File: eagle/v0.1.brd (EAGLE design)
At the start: 20 x 62.2 mm, 12 parts, among them IC1 74LS595N

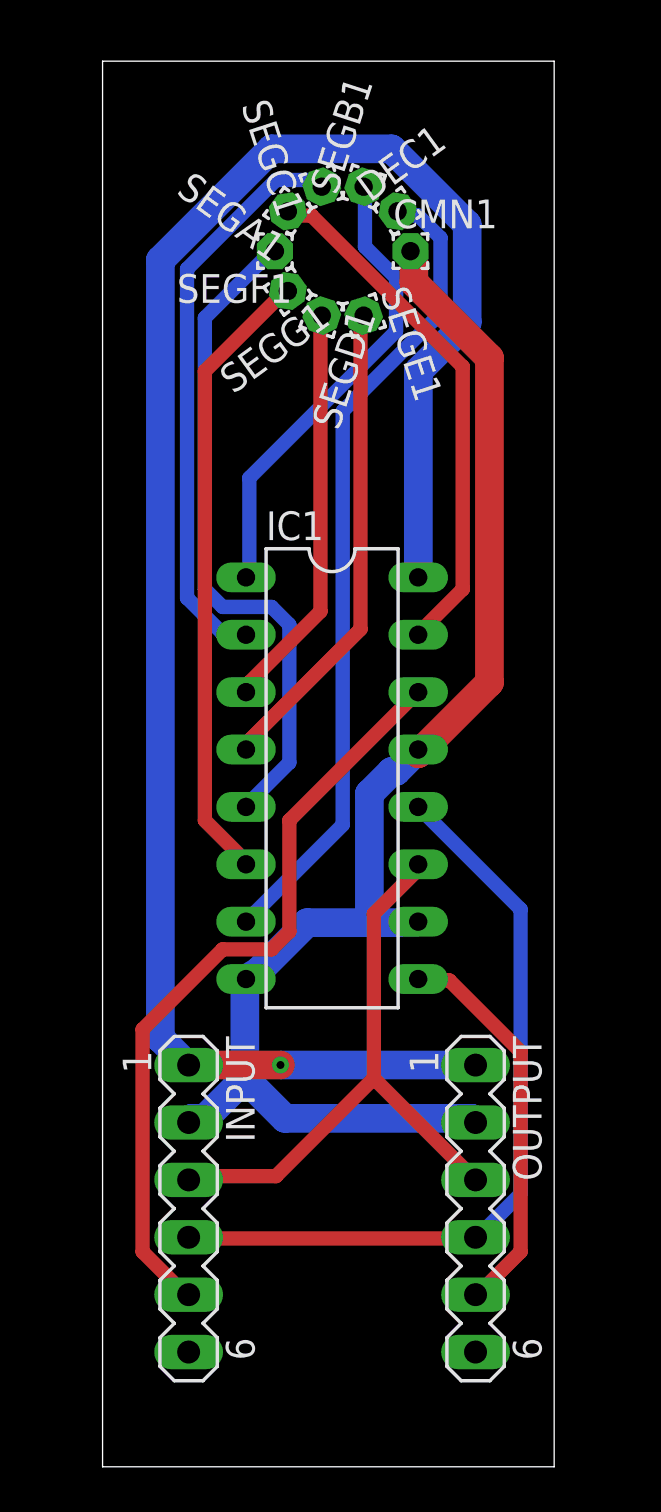
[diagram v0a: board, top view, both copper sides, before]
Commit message: v0.1 as sent to fab
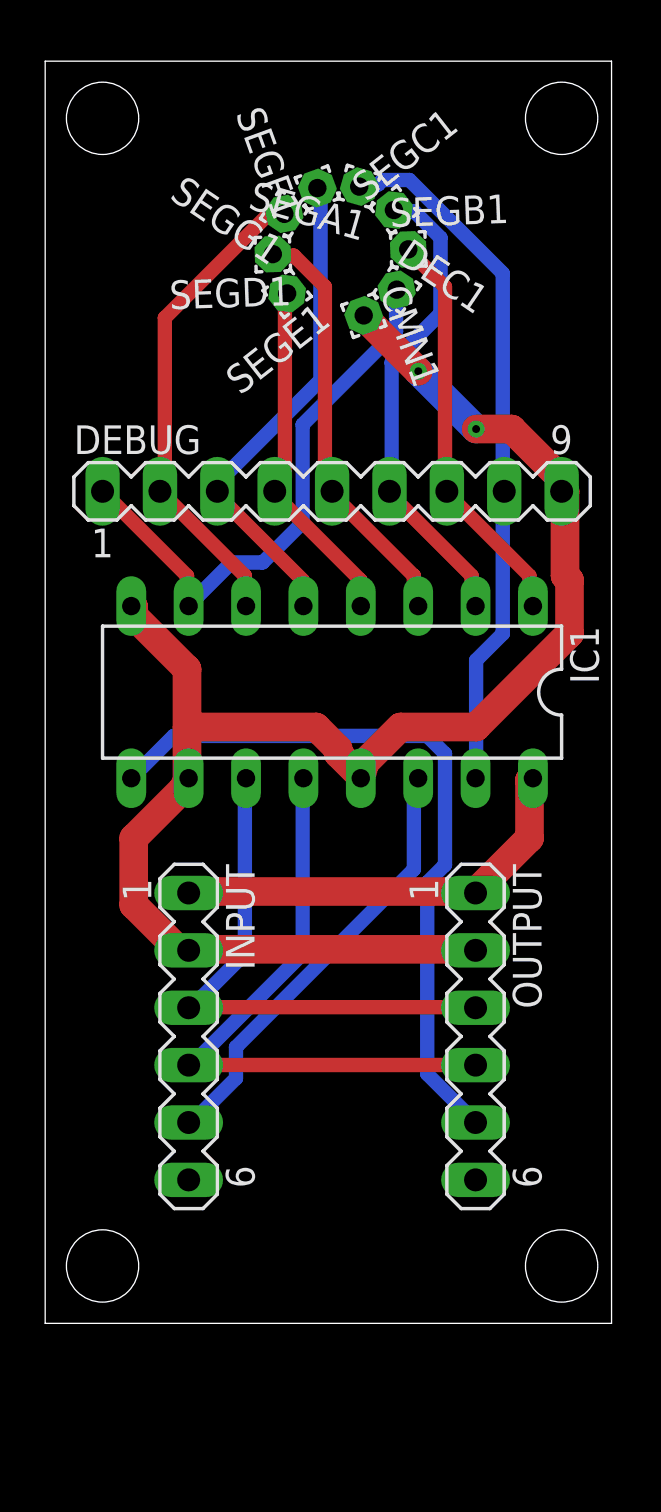
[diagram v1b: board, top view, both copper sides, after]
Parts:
- added DEBUG: (no value), con-lstb:MA09-1
- moved INPUT 7.62 mm to (43.2, 15.2)
- moved OUTPUT 7.62 mm to (55.9, 15.2)
- moved IC1 3.81 mm to (49.5, 30.5), turned to 180 degrees
- moved SEGE1 3.53 mm to (47.5, 48.1), turned to 218 degrees
- moved CMN1 3.52 mm to (50.9, 47.2), turned to 290 degrees
- moved SEGD1 3.48 mm to (46.9, 49.9), turned to 182 degrees
- moved DEC1 3.47 mm to (52.4, 48.3), turned to 326 degrees
- moved SEGG1 3.42 mm to (47.4, 51.7), turned to 146 degrees
- moved SEGB1 3.41 mm to (52.9, 50.1), turned to 2 degrees
- moved SEGF1 3.37 mm to (48.9, 52.8), turned to 110 degrees
- moved SEGC1 3.36 mm to (52.3, 51.8), turned to 38 degrees
- moved SEGA1 3.34 mm to (50.7, 52.9), turned to 164 degrees
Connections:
- net GND: now also DEBUG.9
- net N$1: now also DEBUG.8
- net N$2: now also DEBUG.7
- net N$3: now also DEBUG.6
- net N$4: now also DEBUG.5
- net N$5: now also DEBUG.4
- net N$6: now also DEBUG.3
- net N$7: now also DEBUG.2
- net N$8: now also DEBUG.1
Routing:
- net VCC: track 82.4 -> 18.9 mm, vias 1 -> 0
- net N$9: track 17.6 -> 32.5 mm
- net RX: track 34.0 -> 19.6 mm
- net N$8: track 36.2 -> 25.3 mm
- net GND: track 61.3 -> 71.0 mm, vias 0 -> 2
- net N$1: track 23.3 -> 31.1 mm
- net N$6: track 29.6 -> 22.3 mm
- net RCK: track 34.6 -> 27.6 mm
- net N$7: track 27.7 -> 21.6 mm
- net N$5: track 21.5 -> 15.8 mm
- net N$3: track 25.6 -> 21.6 mm
- net SCK: track 26.8 -> 24.0 mm
- net N$2: track 20.7 -> 18.2 mm
- net N$4: track 18.1 -> 19.0 mm
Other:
- board size 20 x 62.2 mm -> 25.1 x 55.9 mm
